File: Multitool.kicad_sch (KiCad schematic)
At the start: 8 parts, among them SW1 SW_Push

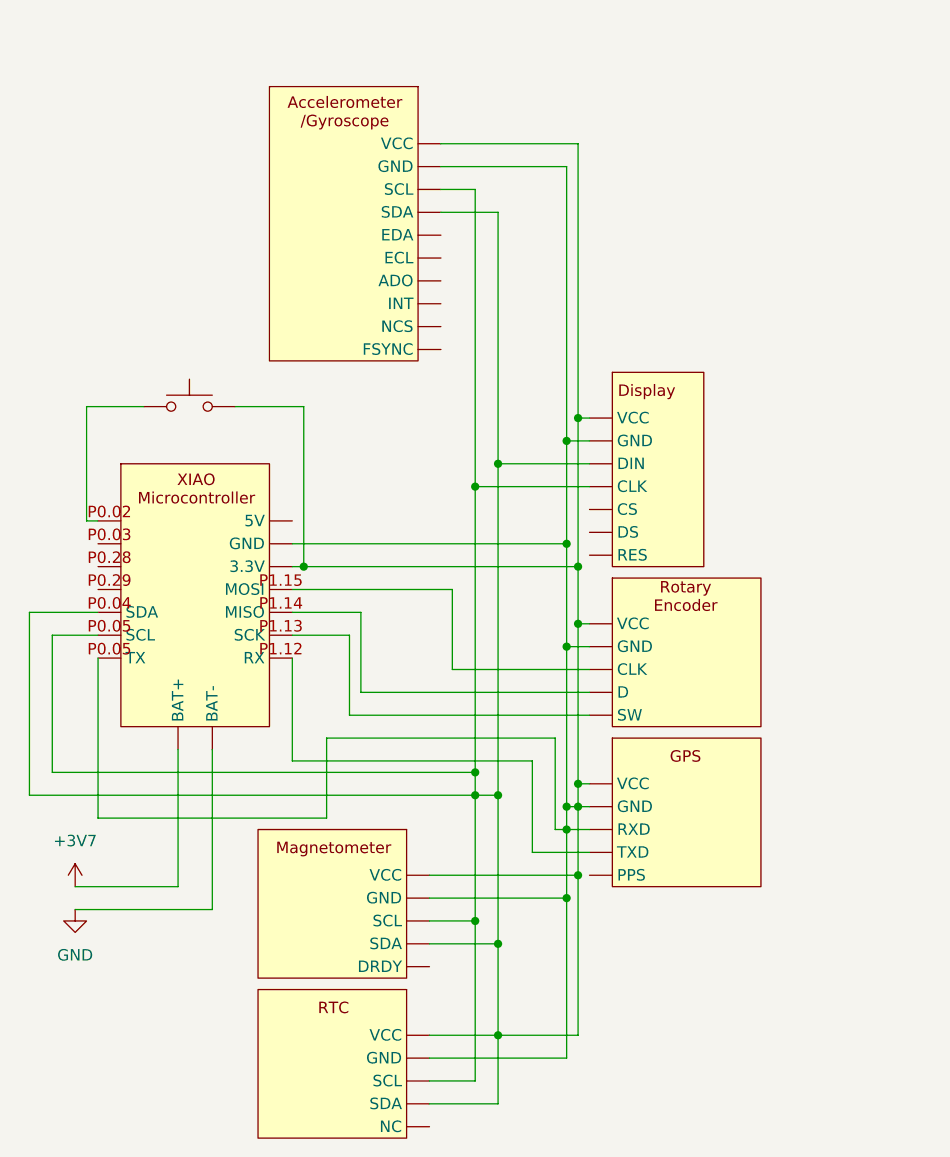
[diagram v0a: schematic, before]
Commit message: Edit schematic
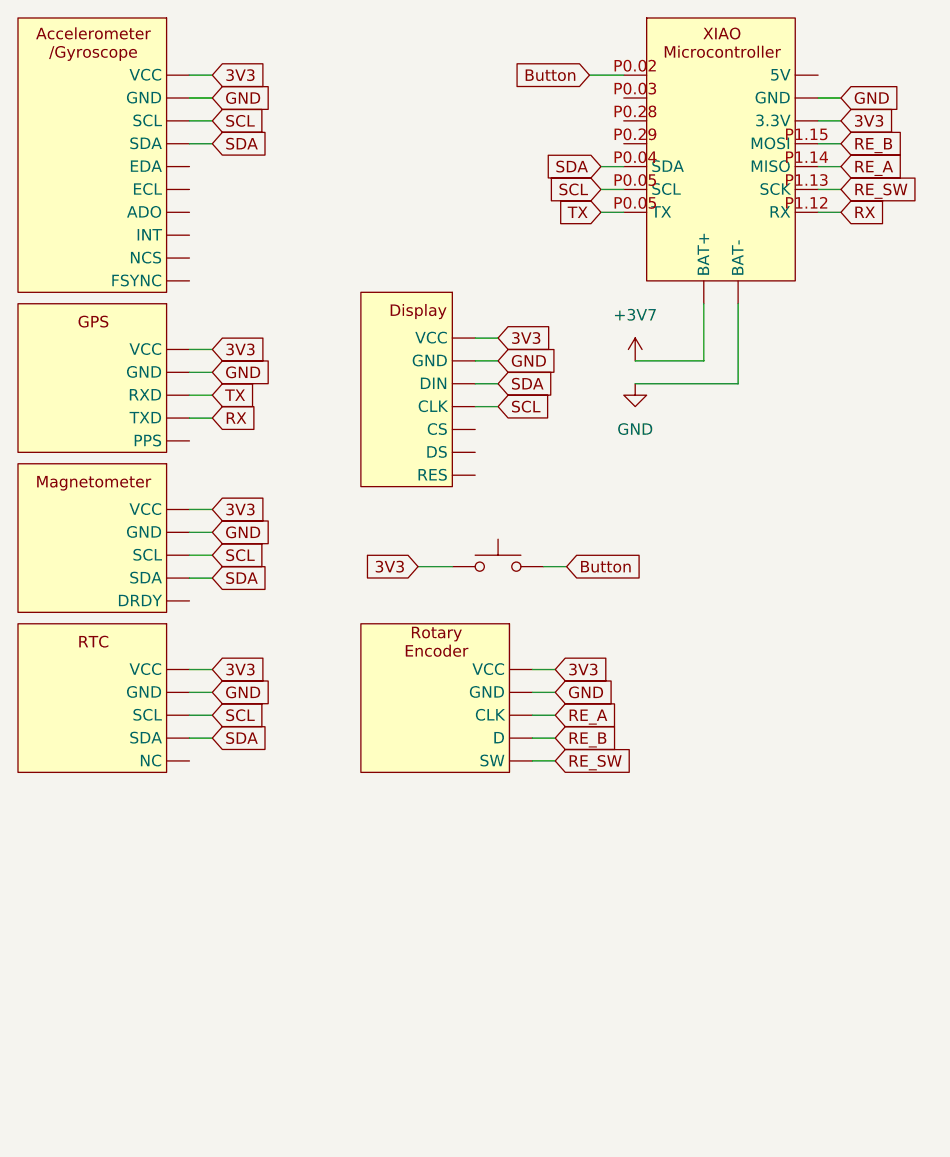
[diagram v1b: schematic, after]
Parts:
- removed SW1: SW_Push, symbol Switch:SW_Push
- removed U1: ~, symbol New_Library:Microcontroller
- removed U2: ~, symbol New_Library:Accelerometer
- removed U3: ~, symbol New_Library:Display
- removed U4: ~, symbol New_Library:GPS
- removed U5: ~, symbol New_Library:Magnetometer
- removed U6: ~, symbol New_Library:RotaryEncoder
- removed U7: ~, symbol New_Library:RTC
- added SW2: SW_Push, symbol Switch:SW_Push
- added U10: ~, symbol New_Library:Accelerometer
- added U11: ~, symbol New_Library:GPS
- added U12: ~, symbol New_Library:RotaryEncoder
- added U13: ~, symbol New_Library:Magnetometer
- added U14: ~, symbol New_Library:RTC
- added U8: ~, symbol New_Library:Microcontroller
- added U9: ~, symbol New_Library:Display
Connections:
- net +3V7: now also U8. (3.3V)
- net GND: now also U10. (FSYNC), U11. (PPS), U12. (SW), U13. (DRDY), U14. (NC), U8. (3.3V), U9. (RES)
- new net 3V3: SW2.1, U10. (FSYNC), U11. (PPS), U12. (SW), U13. (DRDY), U14. (NC), U8. (3.3V), U9. (RES)
- new net Button: SW2.2, U8.P0.02
- new net RE_A: U12. (SW), U8.P1.14 (MISO)
- new net RE_B: U12. (SW), U8.P1.15 (MOSI)
- new net RE_SW: U12. (SW), U8.P1.13 (SCK)
- new net RX: U11. (PPS), U8.P1.12 (RX)
- new net SCL: U10. (FSYNC), U13. (DRDY), U14. (NC), U8.P0.05 (TX), U9. (RES)
- new net SDA: U10. (FSYNC), U13. (DRDY), U14. (NC), U8.P0.04 (SDA), U9. (RES)
- new net TX: U11. (PPS), U8.P0.05 (TX)
